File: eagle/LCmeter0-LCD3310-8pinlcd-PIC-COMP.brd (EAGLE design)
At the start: 50.8 x 63.2 mm, 29 parts, among them K1 DS2Y

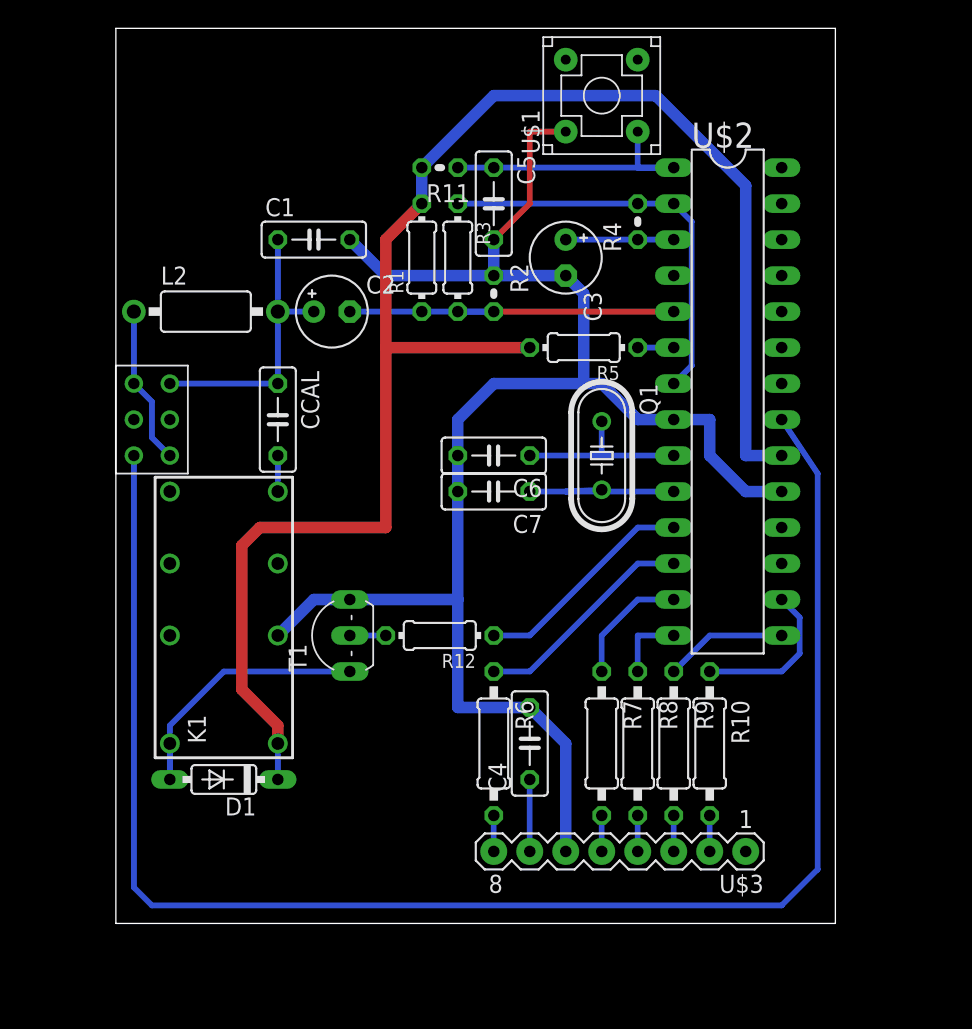
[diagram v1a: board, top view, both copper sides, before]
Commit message: ...
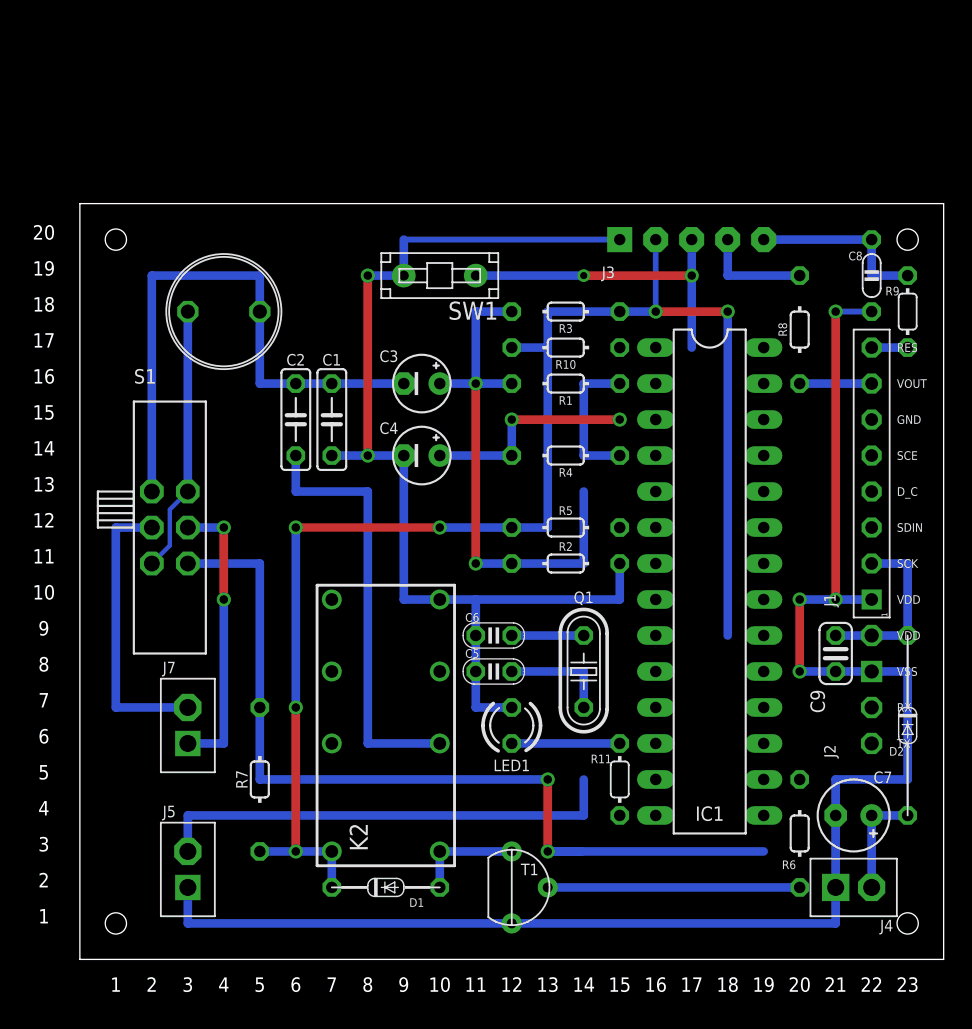
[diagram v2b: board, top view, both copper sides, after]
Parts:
- removed CCAL: 1nF, rcl:C050-025X075
- removed K1: DS2Y, relay:DS2Y
- removed L2: 100uH, rcl:IR-2
- removed R12: 4.7k, rcl:0204/7
- removed U$1: PB-SPST, lc-meter:PB-5
- removed U$2: PIC16F876A-X/SP-COMP, lc-meter:DIL28-3
- removed U$3: NOKIA-3310-64X64, lc-meter:1X8
- removed U$4: S-DPDT, lc-meter:DPDT
- added C8: 22pF, c:C050-020X036
- added C9: 100nF, rcl:C025-024X044
- added D2: 1N4148, d:DO34-12V
- added IC1: PIC16F876A-X/SP-COMPDIL28-3/V, mcu:DIL28-3/V
- added J1: SPI-LCD3310, lcd:CONN-LCD3310
- added J2: PIC-UART, pinconn:PIC-UART
- added J3: PIC-ICSP, pinconn:PIC-ICSP
- added J4: J4, pinconn:CONN-2P
- added J5, J7: CONN-2P2P/V, pinconn:CONN-2P-V
- added K2: DS2Y, relay:DS2Y
- added L1: 68μH, r:L-09R
- added LED1: TLLG4400, led:LED3MM
- added S1: SL-SW-2P-2T-H, sw:SLSW-2P2T-H
- added SW1: PB-1P-1T, sw:PB-1P1T
- C1: device rcl:C050-025X075 -> c:C050-025X060
- C2: value 10uF -> 1nF; device rcl:E2,5-5 -> c:C050-025X060
- C3: value 10uF -> 10μF; device rcl:E2,5-5 -> c:E2,5-4
- C4: value 220nF -> 10μF; device rcl:C050-025X075 -> c:E2,5-4
- C5: value 1nF -> 33pF; device rcl:C050-025X075 -> c:C025-020X036
- C6: value 22pF -> 33pF; device rcl:C050-025X075 -> c:C025-020X036
- C7: value 22pF -> 100μF; device rcl:C050-025X075 -> c:E2,5-5
- D1: device diode:DO35-7 -> d:DO34-7
- Q1: value (none) -> 20MHz; device crystal:HC49/S -> q:HC49
- R1, R3: value 100k -> 100kΩ; device rcl:0204/7 -> r:0202/7
- R10: value 3.3k -> 4.7kΩ; device rcl:0207/10 -> r:0202/7
- R11: value 4.7k -> 1k; device rcl:0204V -> r:0202/5-V
- R2: value 100k -> 100kΩ; device rcl:0204V -> r:0202/7
- R4: value 47k -> 47kΩ; device rcl:0204V -> r:0202/7
- R5: value 4.7k -> 4.7kΩ; device rcl:0204/7 -> r:0202/7
- R6: value 3.3k -> 10k; device rcl:0207/10 -> r:0202/7-V
- R7: value 3.3k -> 10kΩ; device rcl:0207/10 -> r:0202/10
- R8: value 3.3k -> 100; device rcl:0207/10 -> r:0202/7
- R9: value 3.3k -> 100; device rcl:0207/10 -> r:0202/5-V
- T1: value (none) -> BC547; device transistor:TO92-CBE -> t:TO92-CBE-A
- moved R11 45.0 mm to (35.6, 10.2), turned to 0 degrees
- moved R9 34.7 mm to (55.9, 43.2), turned to 0 degrees
- moved C7 34.2 mm to (52.1, 7.62), turned to 0 degrees
- moved C5 33.0 mm to (25.4, 17.8), turned to 0 degrees
- moved R8 31.4 mm to (48.3, 41.9)
- moved R10 29.7 mm to (31.8, 40.6), turned to 0 degrees
- moved R7 24.3 mm to (10.2, 10.2), turned to 0 degrees
- moved R6 22.5 mm to (48.3, 6.35), turned to 180 degrees
- moved C4 22.2 mm to (20.3, 33.0), turned to 0 degrees
- moved T1 21.1 mm to (27.9, 2.54), turned to 0 degrees
- moved R2 19.7 mm to (31.8, 25.4), turned to 180 degrees
- moved R4 17.3 mm to (31.8, 33.0), turned to 0 degrees
- moved Q1 15.3 mm to (33.0, 17.8), turned to 0 degrees
- moved C3 14.5 mm to (20.3, 38.1), turned to 0 degrees
- moved D1 13.7 mm to (19.1, 2.54), turned to 0 degrees
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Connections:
- removed net +3V3: U$3.1
- removed net +5V: D1.C, K1.1, R1.2, R11.2, R5.2, U$2.20
- removed net L/C: U$2.21, U$4.2-3
- removed net N$13: R8.2, U$3.4
- removed net N$14: R7.2, U$3.5
- removed net N$15: R6.2, U$3.8
- removed net N$16: C4.1, U$3.7
- removed net N$17: R3.1, R4.2, U$2.2, U$2.7
- removed net N$19: R12.2, T1.B
- removed net N$20: D1.A, K1.16, T1.C
- removed net N$21: CCAL.2, K1.8
- removed net N$23: C1.1, C2.+, CCAL.1, L2.2, U$4.1-2
- removed net N$24: L2.1, U$4.1-3, U$4.2-2
- removed net N$3: R8.1, U$2.14
- removed net N$4: R9.1, U$2.15
- removed net RA1: C3.+, R4.1, U$2.3
- removed net RA3: C2.-, R1.1, R2.2, R3.2, U$2.5
- removed net RELAY: R12.1, U$2.11
- new net /LC: IC1.15, R7.2, S1.6
- new net /MCLR: J3.3, R10.2, SW1.2
- new net /RELAY: D1.A, K2.1, T1.C
- new net A0: IC1.2, IC1.7, R1.2, R4.2
- new net A1: C4.+, IC1.3, R4.1
- new net A3: C3.+, IC1.5, R1.1, R2.2, R3.1
- new net A4: IC1.6, R5.1
- new net C2_CON: C2.2, K2.4
- new net D4: IC1.25, J1.SCE
- new net D5: IC1.26, J1.GND
- new net D6: IC1.27, J1.VOUT, R8.2
- new net D7: IC1.28, J1.RES, R9.2
- new net E: IC1.24, J1.D_C
- new net FREQ: IC1.11, IC1.13, J5.2
- new net M+: J7.2, S1.2
- new net M-: J7.1, S1.5
- new net N$7: L1.P$1, S1.3, S1.4
- new net OSC1: C6.2, IC1.8, Q1.2
- new net OSC2: C5.2, IC1.9, Q1.1
- new net PGC: J3.4, R8.1
- new net PGD: C8.2, J3.5, R9.1
- new net RS: IC1.23, J1.SDIN
- new net VCC: C9.1, D1.C, D2.C, IC1.4, J1.SCK, J2.20, J3.2, K2.16, R10.1, R3.2, R5.2, R7.1
- net GND: now also C4.-, C5.1, C6.1, C7.-, C8.1, C9.2, IC1.10, IC1.19, J1.VDD, J2.19, J3.1, J4.1, J5.1, K2.8, LED1.K, SW1.1; no longer C3.-, C4.2, C5.2, C6.2, C7.2, K1.4, U$1.4, U$2.19, U$2.8, U$3.6
- net N$1: now also LED1.A, R11.1; no longer R6.1, U$2.12
- net N$10: now also IC1.17, J2.17; no longer C6.1, Q1.1, U$2.9
- net N$11: now also IC1.21, IC1.22; no longer R10.2, U$3.2
- net N$12: now also C7.+, D2.A, J4.2; no longer R9.2, U$3.3
- net N$2: now also C1.1, C2.1, C3.-, L1.P$2, S1.1; no longer R7.1, U$2.13
- net N$5: now also IC1.14, R11.2; no longer R10.1, U$2.16
- net N$6: now also R6.2, T1.B; no longer R5.1, U$2.6
- net N$8: now also IC1.16, R6.1; no longer C5.1, R11.1, U$1.2, U$2.1
- net N$9: now also IC1.18, J2.18; no longer C7.1, Q1.2, U$2.10
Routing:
- net VCC: track 0.00 -> 119.4 mm, vias 0 -> 6
- net +5V: track 114.0 -> 0.00 mm
- net L/C: track 112.8 -> 0.00 mm
- net GND: track 117.1 -> 188.0 mm, vias 0 -> 6
- net /LC: track 0.00 -> 63.3 mm, vias 0 -> 2
- net A3: track 0.00 -> 38.1 mm, vias 0 -> 2
- net FREQ: track 0.00 -> 33.0 mm
- net N$2: track 8.67 -> 40.6 mm
- net C2_CON: track 0.00 -> 30.5 mm
- net N$17: track 29.0 -> 0.00 mm
- net RA3: track 25.4 -> 0.00 mm
- net /MCLR: track 0.00 -> 22.9 mm, vias 0 -> 2
- net N$20: track 20.6 -> 0.00 mm
- net M-: track 0.00 -> 20.3 mm, vias 0 -> 2
- net M+: track 0.00 -> 20.3 mm
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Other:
- board size 50.8 x 63.2 mm -> 61 x 53.3 mm
- board text added: "1"
- board text added: "10"
- board text added: "11"
- board text added: "12"
- board text added: "13"
- board text added: "14"
- board text added: "15"
- board text added: "16"
- board text added: "17"
- board text added: "18"
- board text added: "19"
- board text added: "2"
- board text added: "20"
- board text added: "21"
- board text added: "22"
- board text added: "23"
- board text added: "3"
- board text added: "4"
- board text added: "5"
- board text added: "6"
- board text added: "7"
- board text added: "8"
- board text added: "9"
